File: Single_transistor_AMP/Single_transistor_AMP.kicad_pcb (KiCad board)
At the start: 2 copper layers, 0 parts

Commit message: 1.4
Izveidots PCB dizains, kā arī papildināta shēma
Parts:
- added C1: 20uF, Capacitors_THT:CP_Axial_L18.0mm_D8.0mm_P25.00mm_Horizontal, F.Cu at (115.6, 85.1)
- added C2: 50uF, Capacitors_THT:CP_Axial_L21.0mm_D8.0mm_P28.00mm_Horizontal, F.Cu at (133.3, 94.0)
- added C3: 20uF, Capacitors_THT:CP_Axial_L18.0mm_D8.0mm_P25.00mm_Horizontal, F.Cu at (85.1, 113.0)
- added J1: Conn_01x02, Connectors:Banana_Jack_2Pin, F.Cu at (91.4, 120.7)
- added P1: Signal_In, Connectors_Terminal_Blocks:TerminalBlock_Altech_AK300-2_P5.00mm, F.Cu at (146.1, 111.8)
- added P2: Signal_Out, Connectors_Terminal_Blocks:TerminalBlock_Altech_AK300-2_P5.00mm, F.Cu at (146.1, 97.8)
- added Q1: BC548, TO_SOT_Packages_THT:TO-92_Molded_Narrow, F.Cu at (99.1, 85.1)
- added R1: 22k, Resistors_THT:R_Axial_DIN0516_L15.5mm_D5.0mm_P20.32mm_Horizontal, F.Cu at (104.1, 111.8)
- added R2: 6.8k, Resistors_THT:R_Axial_DIN0516_L15.5mm_D5.0mm_P20.32mm_Horizontal, F.Cu at (113.0, 91.4)
- added R3: 4.7k, Resistors_THT:R_Axial_DIN0516_L15.5mm_D5.0mm_P20.32mm_Horizontal, F.Cu at (95.2, 111.8)
- added R4: 1.8k, Resistors_THT:R_Axial_DIN0516_L15.5mm_D5.0mm_P20.32mm_Horizontal, F.Cu at (121.9, 91.4)
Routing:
- net Net-(C3-Pad1): track 0.00 -> 67.3 mm
- net GND: track 0.00 -> 65.1 mm
- net Net-(C2-Pad1): track 0.00 -> 40.5 mm
- net Net-(C1-Pad2): track 0.00 -> 30.4 mm
- net Net-(C1-Pad1): track 0.00 -> 25.5 mm
- net Net-(C3-Pad2): track 0.00 -> 19.5 mm
- net +12V: track 0.00 -> 19.4 mm
- added copper zone on B.Cu, net GND
- added copper zone on F.Cu, net GND
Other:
- board outline added: 74.9 x 45.7 mm

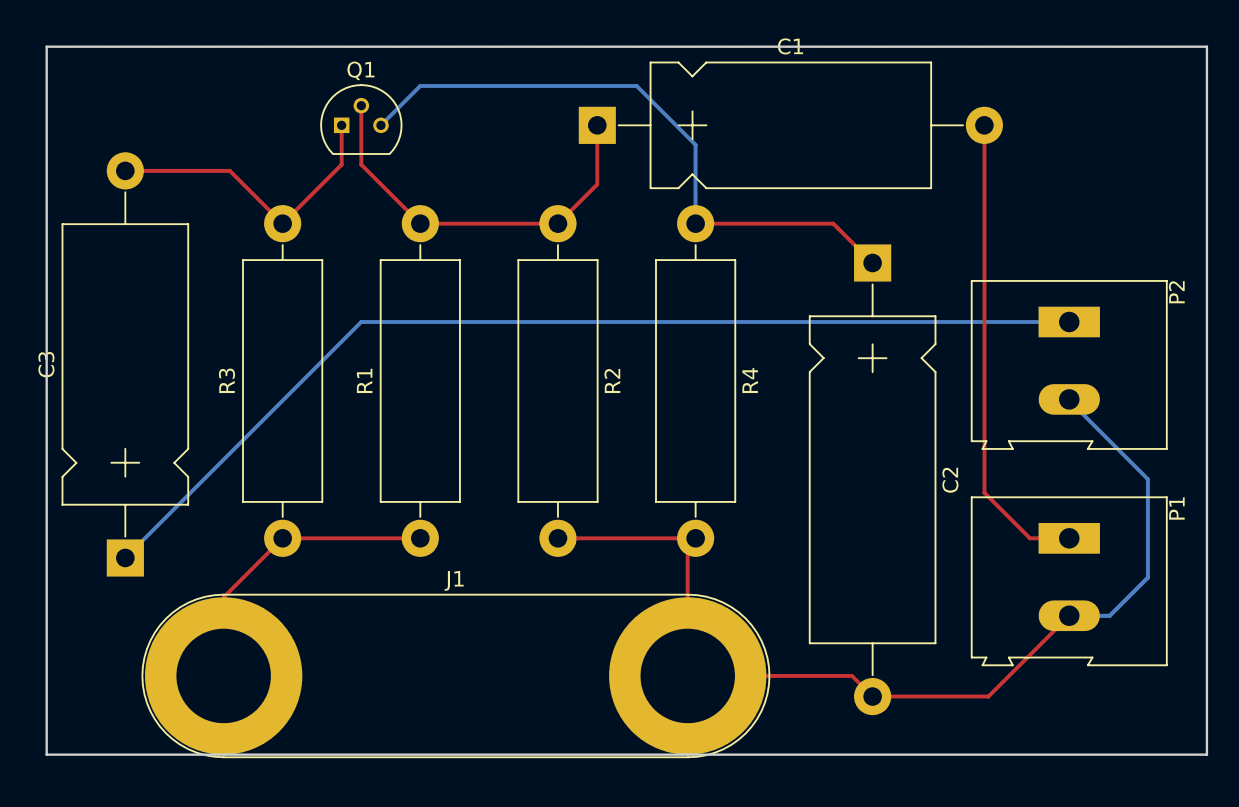
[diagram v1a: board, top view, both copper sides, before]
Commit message: 1.7
1.6 Tika dizainēta plate ar tās slāņiem.
1.7 Tiek izveidoti gerber faili.
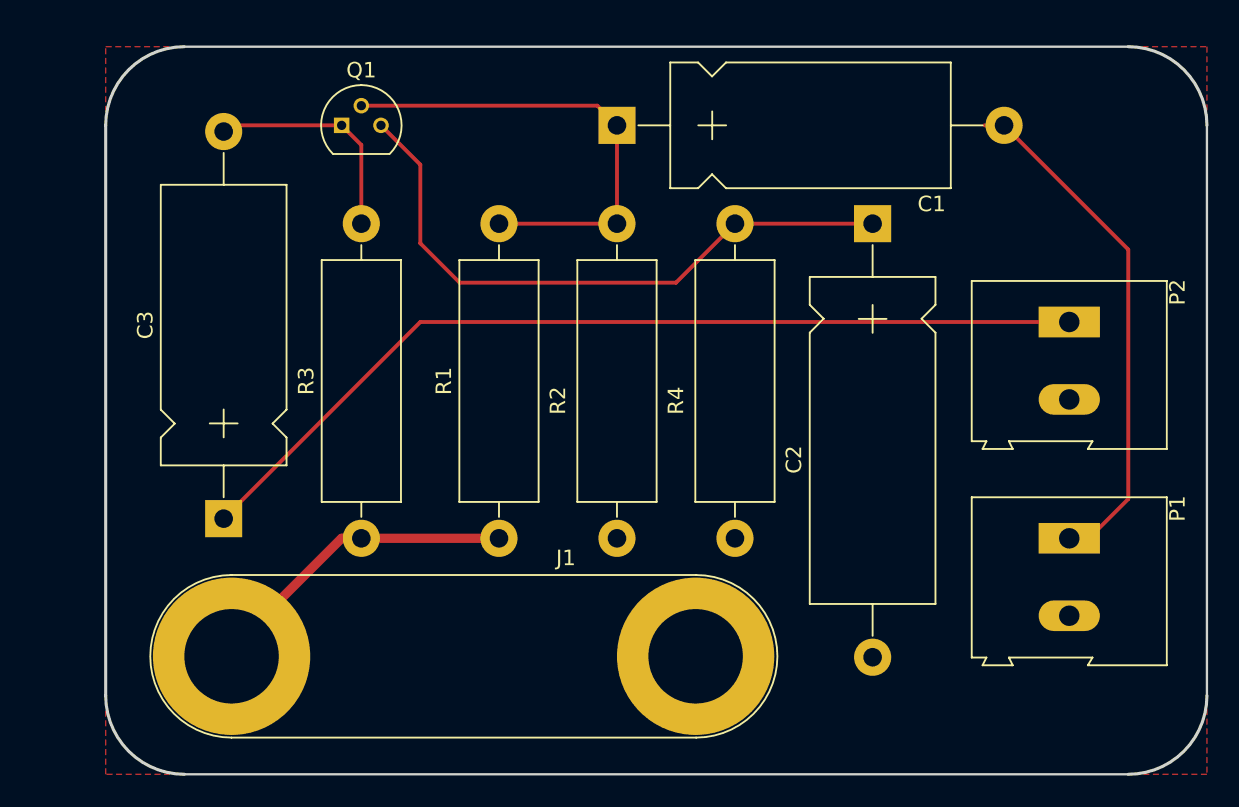
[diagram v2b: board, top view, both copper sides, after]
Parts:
- moved C3 6.84 mm to (91.4, 110.5)
- moved R1 5.08 mm to (109.2, 111.8)
- moved R3 5.08 mm to (100.3, 111.8)
- moved R2 3.81 mm to (116.8, 91.4)
- moved C2 2.54 mm to (133.3, 91.4)
- moved R4 2.54 mm to (124.5, 91.4)
- moved J1 1.37 mm to (92.0, 119.4)
- moved C1 1.27 mm to (116.8, 85.1)
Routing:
- net GND: track 65.1 -> 0.08 mm
- net Net-(C3-Pad1): track 67.3 -> 59.9 mm
- net Net-(C1-Pad1): track 25.5 -> 31.0 mm
- net Net-(C3-Pad2): track 19.5 -> 14.7 mm
- net Net-(C1-Pad2): track 30.4 -> 34.0 mm
- net +12V: track 19.4 -> 20.9 mm
- removed copper zone on B.Cu, net GND
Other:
- board size 74.9 x 45.7 mm -> 71.1 x 47 mm
- net class Power: trace_width 0.3 -> 0.6
